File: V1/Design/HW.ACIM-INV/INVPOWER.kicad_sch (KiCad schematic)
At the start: 55 parts, among them J1 AC POWER INPUT, M4 470V/1.2kA, M5 470V/1.2kA, M6 470V/1.2kA, M7 470V/1.2kA, Q10 20V/1A, Q11 20V/1A, U14 LDO 5V±1%, U4 SMPS 16V±2%/0.6A

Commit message: V1 schematic update 15
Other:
- company: TON DUC THANG UNIVERSITY -> (none)
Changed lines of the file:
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@@
 		(date "2024-09-24")
 		(rev "1.0")
-		(company "TON DUC THANG UNIVERSITY")
-		(comment 1 "Schematic Designed by ...")
-		(comment 2 "PCB Designed by ...")
-		(comment 3 "Approved by ...")
 	)
 	(junction

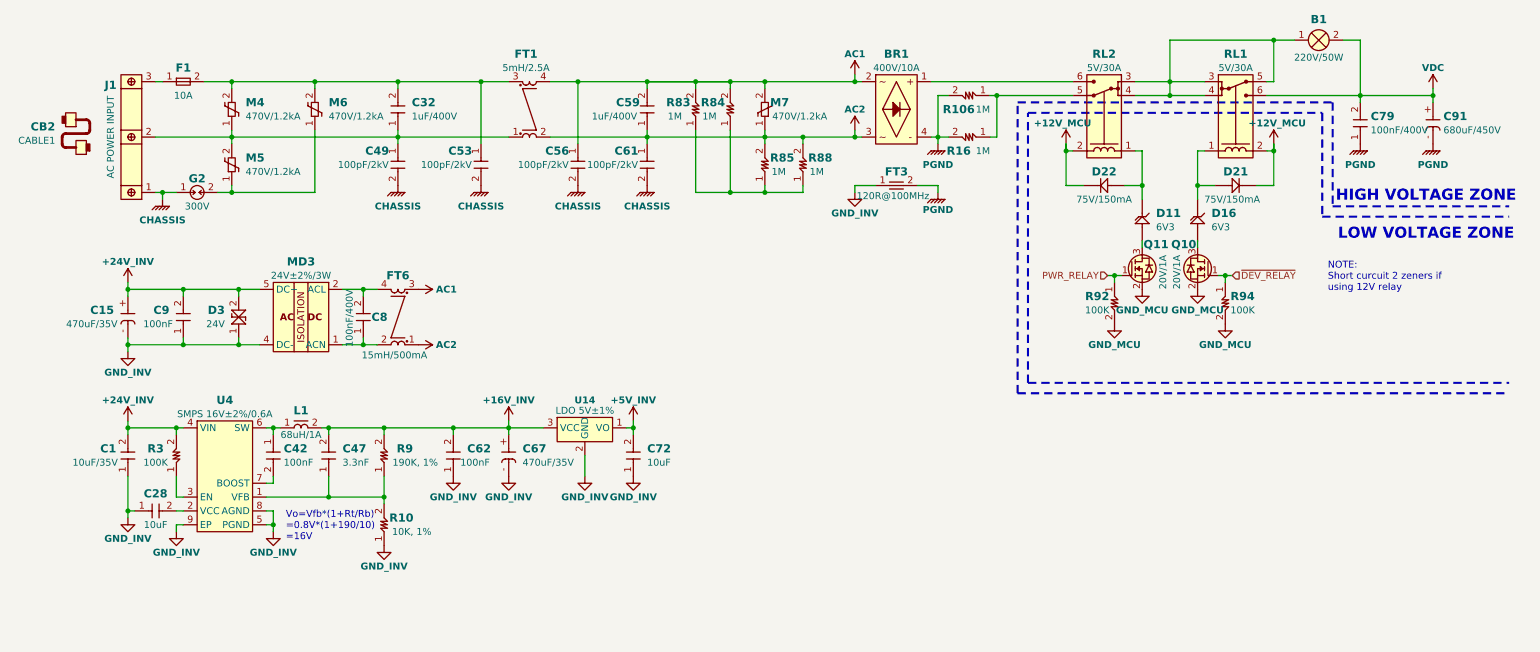
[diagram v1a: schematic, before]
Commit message: V1 schematic update 16
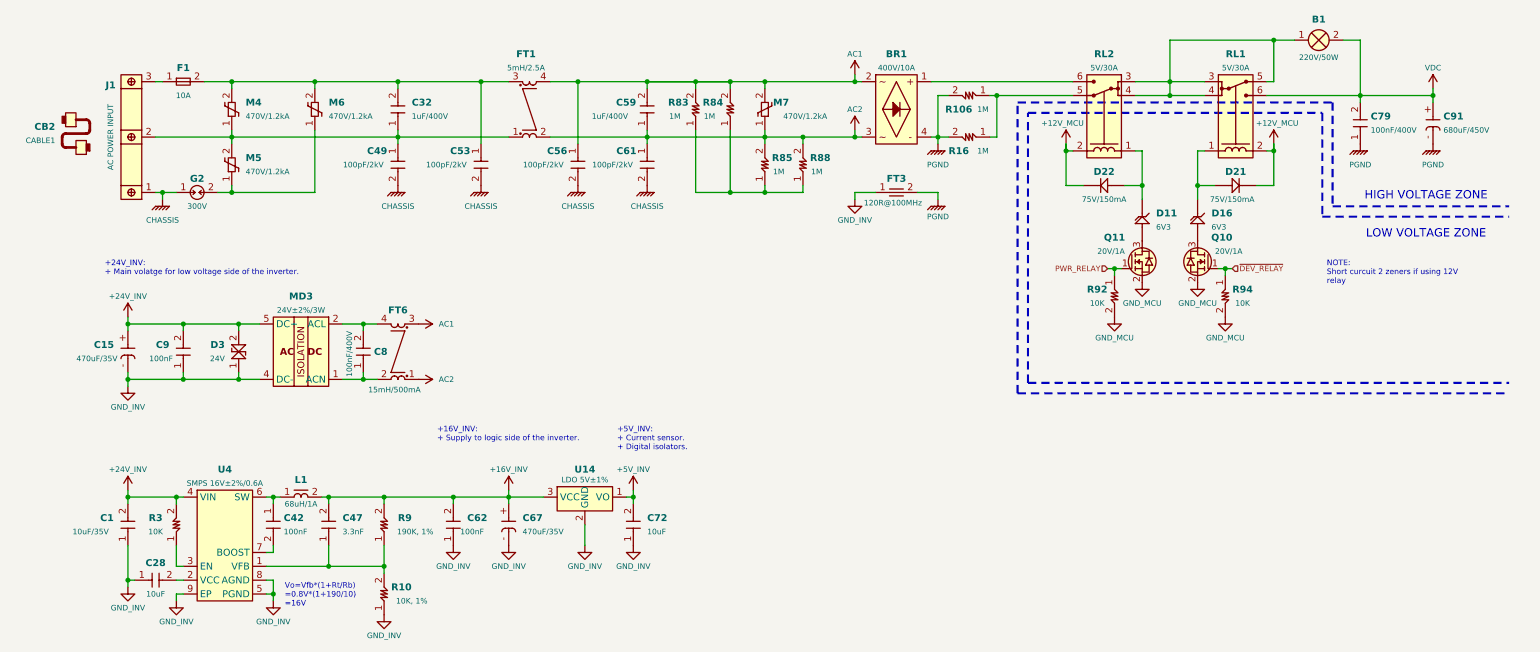
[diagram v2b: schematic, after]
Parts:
- C1: footprint SAMPI:CAP0603 -> SAMPI:CAP1206; MFT Samsung -> (none); MNP CL10A106MQ8NNNC -> (none)
- R3, R92, R94: value 100K -> 10K; MFT YAGEO -> (none); MNP RC0603FR-07100KL -> (none)
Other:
- moved on the sheet: C1, C15, C28, C42, C47, C62, C67, C72, C8, C9, D3, FT3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
